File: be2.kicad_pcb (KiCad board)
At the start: 2 copper layers, 34 parts, among them K1 mini_banana_jack, K2 mini_banana_jack, K3 mini_banana_jack, K4 mini_banana_jack, K5 mini_banana_jack, K6 mini_banana_jack, U1 AD620A, U2 TL082, U3 TL082

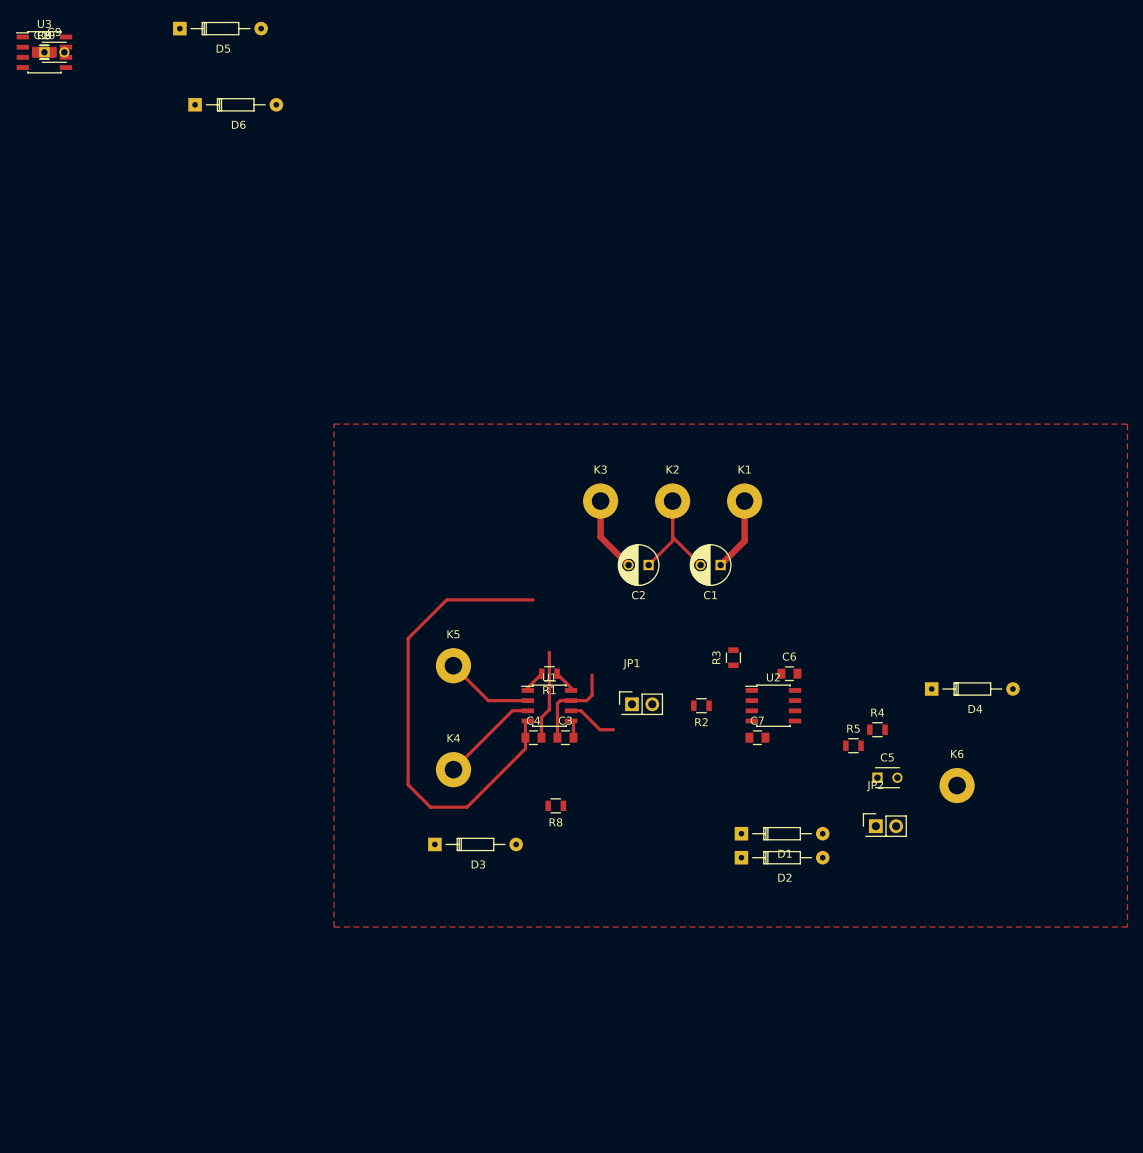
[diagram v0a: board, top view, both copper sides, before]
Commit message: we're routed, fall back!
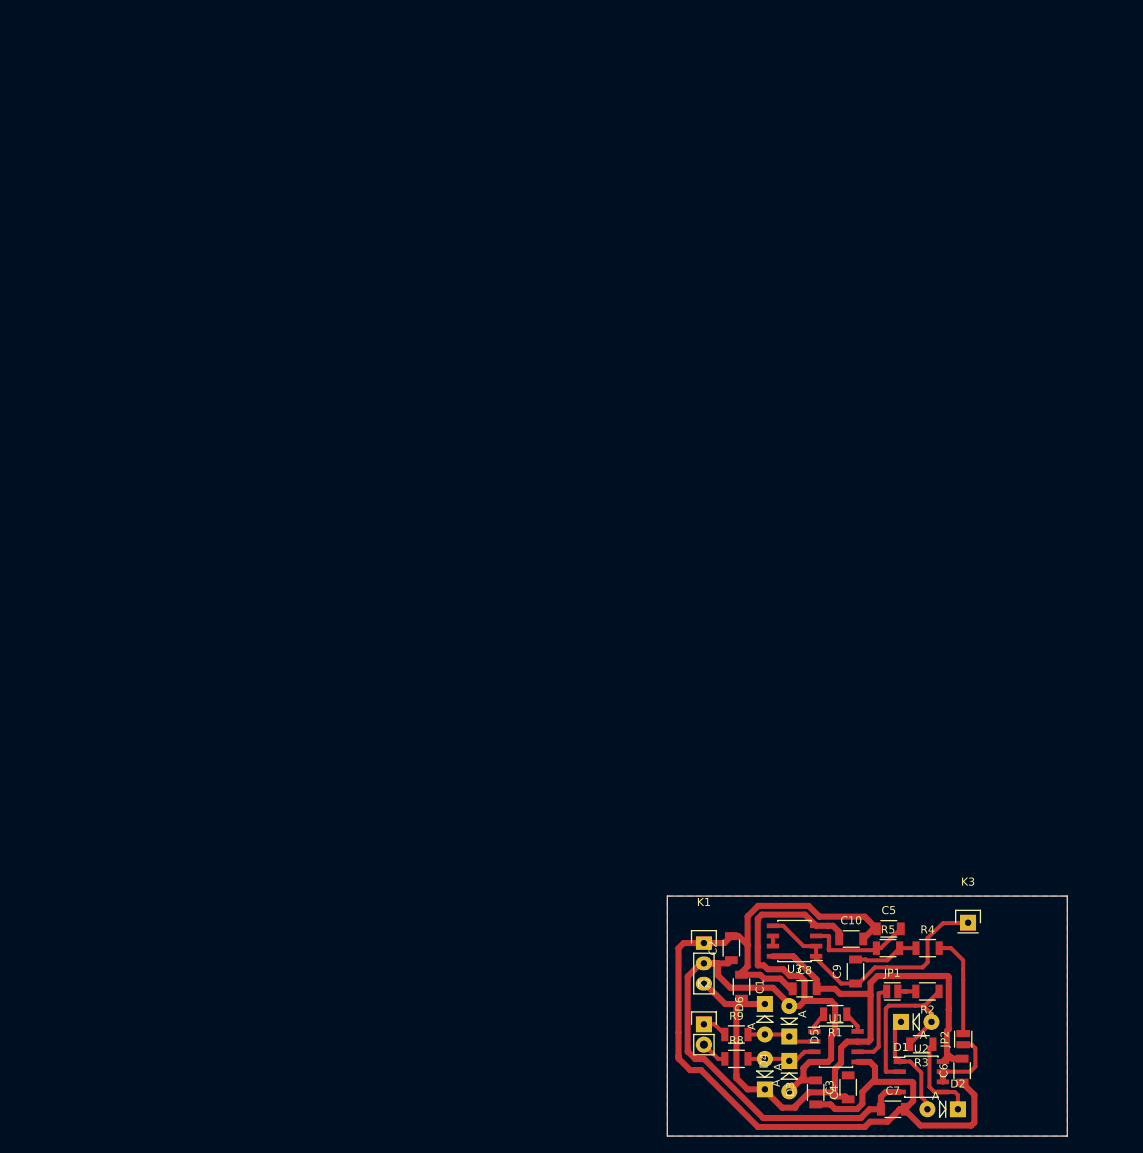
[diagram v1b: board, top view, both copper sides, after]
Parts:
- removed K4, K5, K6: mini_banana_jack, lib:mini_banana_jack_2mm
- C1, C2: value 10u -> 1u; footprint Capacitors_ThroughHole:C_Radial_D5_L6_P2.5 -> Capacitors_SMD:C_1206
- C10, C3, C4, C6, C7, C8: footprint Capacitors_SMD:C_0805 -> Capacitors_SMD:C_1206
- C5, C9: footprint Capacitors_ThroughHole:C_Disc_D3_P2.5 -> Capacitors_SMD:C_1206
- D1, D2, D3, D4, D5, D6: footprint Diodes_ThroughHole:Diode_DO-35_SOD27_Horizontal_RM10 -> lib:Diode_DO-41_SOD81_Vertical_AnodeUp_phelma
- JP1, JP2: footprint Pin_Headers:Pin_Header_Straight_2x01 -> lib:JP_20mil
- K1: value mini_banana_jack -> CONN_01X03; footprint lib:mini_banana_jack_2mm -> lib:Pin_Header_Straight_1x03_phelma
- K2: value mini_banana_jack -> CONN_01X02; footprint lib:mini_banana_jack_2mm -> lib:Pin_Header_Straight_1x02_phelma
- K3: value mini_banana_jack -> CONN_01X01; footprint lib:mini_banana_jack_2mm -> lib:Pin_Header_Straight_1x01_phelma
- R1, R2, R3, R4, R5, R8, R9: footprint Resistors_SMD:R_0805 -> Resistors_SMD:R_1206
- moved C9 153.2 mm to (101.4, 114.9), turned to 90 degrees
- moved C8 150.8 mm to (95.0, 117.1)
- moved R9 150.2 mm to (86.5, 122.8)
- moved C10 149.9 mm to (100.9, 110.8)
- moved D5 147.2 mm to (93.1, 123.0), turned to 90 degrees
- moved U3 145.4 mm to (93.8, 111.1), turned to 180 degrees
- moved D6 133.1 mm to (90.1, 119.0), turned to 270 degrees
- moved K3 69.9 mm to (115.5, 108.8)
- moved K2 65.5 mm to (82.4, 121.5)
- moved C4 56.7 mm to (96.4, 130.0), turned to 270 degrees
- moved C3 56.2 mm to (100.5, 129.4), turned to 90 degrees
- moved U1 55.7 mm to (98.9, 124.3)
- moved R1 55.6 mm to (98.8, 120.2)
- moved K1 55.5 mm to (82.4, 111.3)
- moved C6 54.1 mm to (114.7, 127.3), turned to 90 degrees
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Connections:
- C1 pad 1: VCC -> GND
- C1 pad 2: GND -> VCC
- C2 pad 1: GND -> VSS
- C2 pad 2: VSS -> GND
- K1 pad 1: VCC -> GND
- K2 pad 1: GND -> /in-
- K3 pad 1: VSS -> /mean_out
- U3 pad 2: GND -> /mean_out
- U3 pad 5: GND -> /mean_out
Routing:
- net GND: track 32.1 -> 130.7 mm
- net VCC: track 20.8 -> 92.0 mm
- net VSS: track 67.8 -> 112.0 mm
- net /mean_out: track 0.00 -> 33.5 mm
- net /u2_in-: track 0.00 -> 23.5 mm
- net Net-(C5-Pad2): track 0.00 -> 14.2 mm
- net /u2_out: track 0.00 -> 14.0 mm
- net /mean_in: track 0.00 -> 12.8 mm
- net /neg_out: track 0.00 -> 11.3 mm
- net /neg_out_buff: track 0.00 -> 9.58 mm
- net Net-(C9-Pad2): track 0.00 -> 8.24 mm
- net /in+: track 10.4 -> 3.35 mm
- net /inf+: track 1.94 -> 8.87 mm
- net /diff_out: track 6.28 -> 10.6 mm
- net /inf-: track 4.94 -> 8.66 mm
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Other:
- board outline added: 50 x 30 mm
- net class Default: clearance 0.2 -> 0.3302; trace_width 0.4 -> 0.508
- net class power: clearance 0.4 -> 0.3302; trace_width 0.8 -> 0.762
- rule trace_clearance: 0.2 -> 0.3302
- rule trace_min: 0.2 -> 0.508

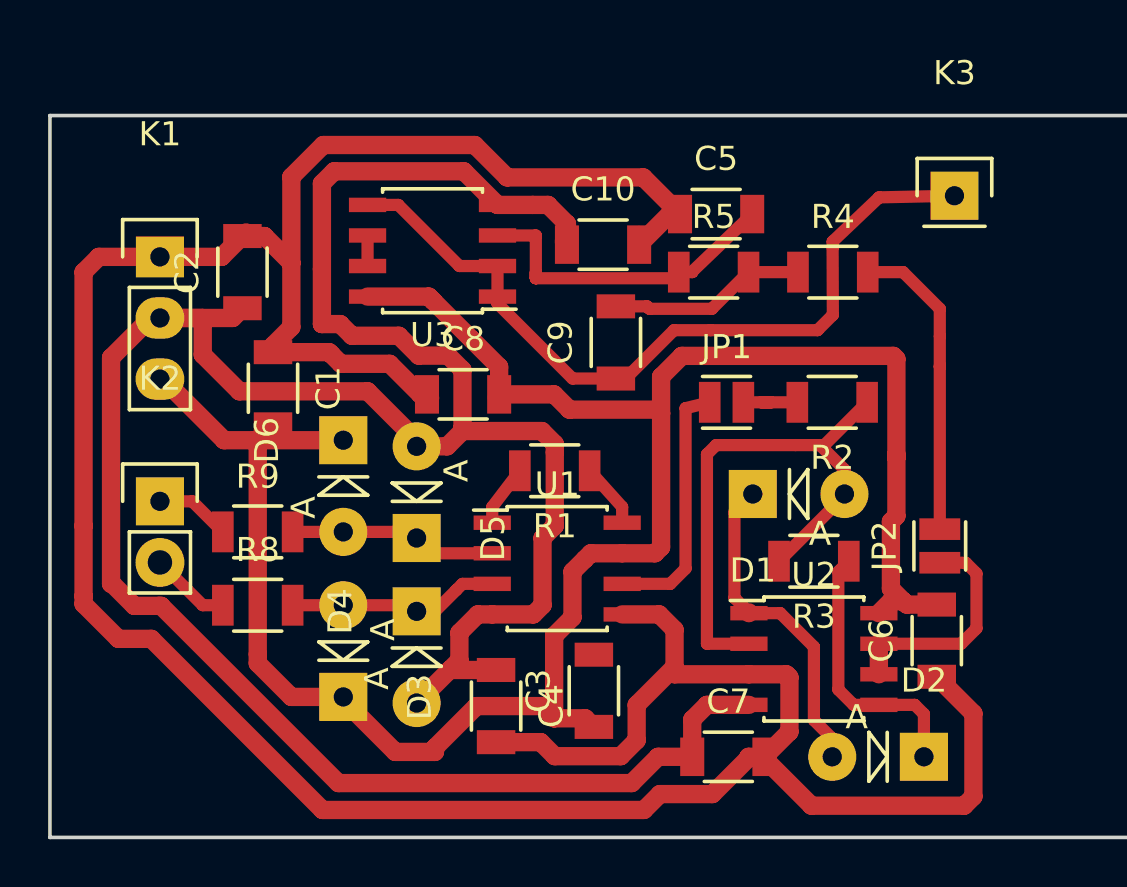
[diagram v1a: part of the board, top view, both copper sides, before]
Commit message: cleaned up the pcb
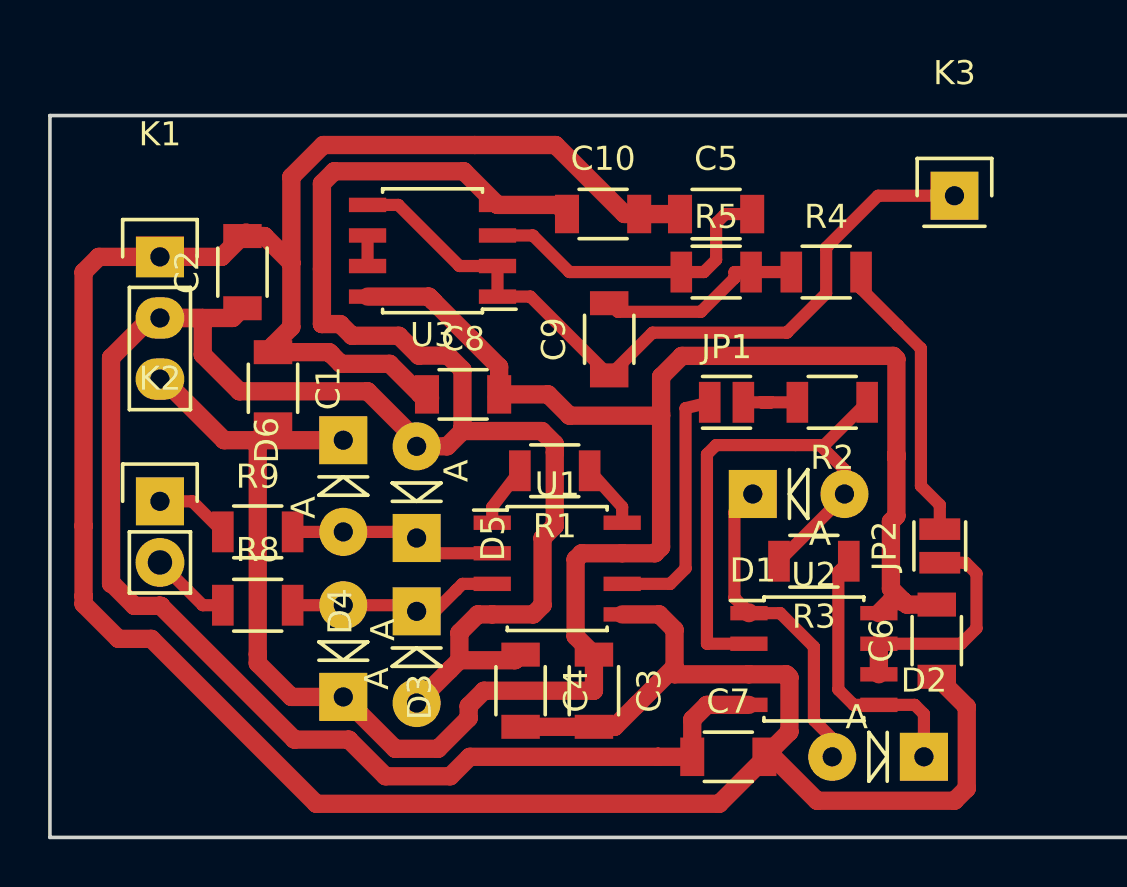
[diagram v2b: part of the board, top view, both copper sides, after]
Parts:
- moved C10 1.27 mm to (100.9, 109.6)
- moved C4 1.20 mm to (97.4, 129.4)
- moved C9 0.31 mm to (101.1, 114.8)
- moved R4 0.28 mm to (110.1, 112.0)
- moved R5 0.10 mm to (105.6, 112.0)
- turned C3 to 270 degrees
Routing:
- net GND: track 130.7 -> 124.4 mm
- net /mean_out: track 33.5 -> 32.3 mm
- net Net-(C5-Pad2): track 14.2 -> 13.1 mm
- net /mean_in: track 12.8 -> 12.0 mm
- net VCC: track 92.0 -> 91.3 mm
- net VSS: track 112.0 -> 111.4 mm
